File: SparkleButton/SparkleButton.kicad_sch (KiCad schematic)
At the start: 5 parts, among them J1 Conn_01x04_Pin, SW1 SW_Push, SW2 SW_Push

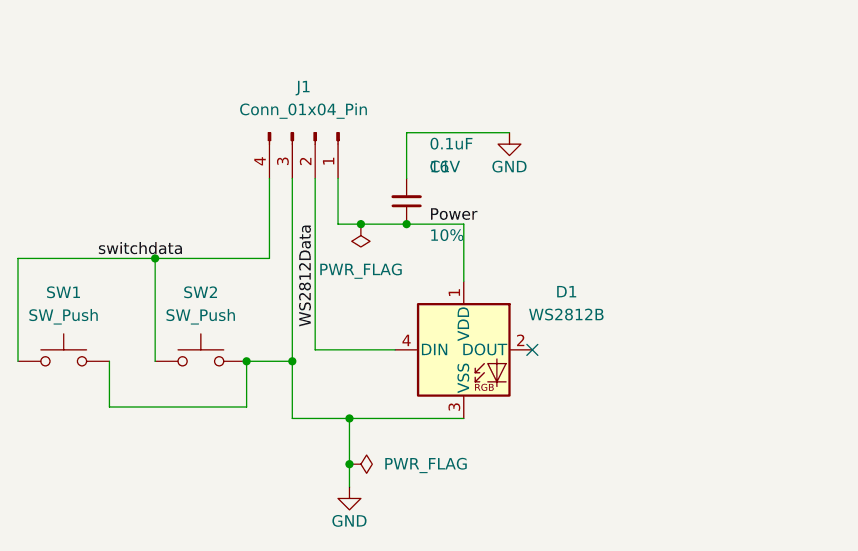
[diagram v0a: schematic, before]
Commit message: updated sparklebutton documentation
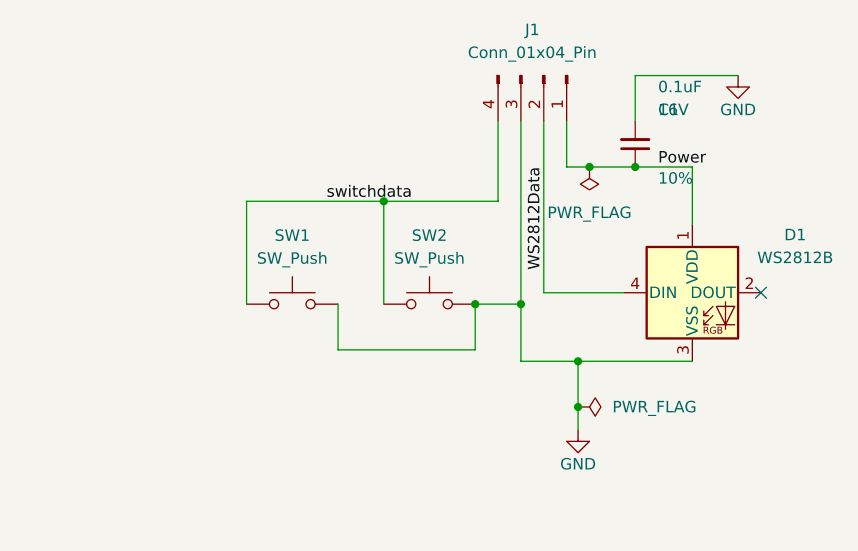
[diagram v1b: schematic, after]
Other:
- company: (none) -> TemuWolverine
- title: (none) -> SparkleButton
- moved on the sheet: C1, D1, J1, SW1, SW2
